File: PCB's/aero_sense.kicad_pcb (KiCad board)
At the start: 2 copper layers, 115 x 58 mm, 115 parts, among them J1 10164228-0201A1RLF, J10 10164227-0205A1RLF, J2 10164228-0201A1RLF, J3 10164228-0201A1RLF, J4 10164228-0201A1RLF, J5 10164227-0205A1RLF, J6 10164227-0205A1RLF, J7 Conn_01x04_Pin, J8 10164227-0205A1RLF, J9 USB4081-03-A_REV0.1, U10 TS3USB221DRCR, U11 KLM8G1GETF-B041, U12 STM32F417IGH6, U2 ICM-42688-P, U3 BMP581, U4 SGP41-D-R4, U5 SHT45-AD1F-R2, U7 SAM-M10Q-00B, U8 BQ25895RTWR, U9 AP2112K-3.3TRG1

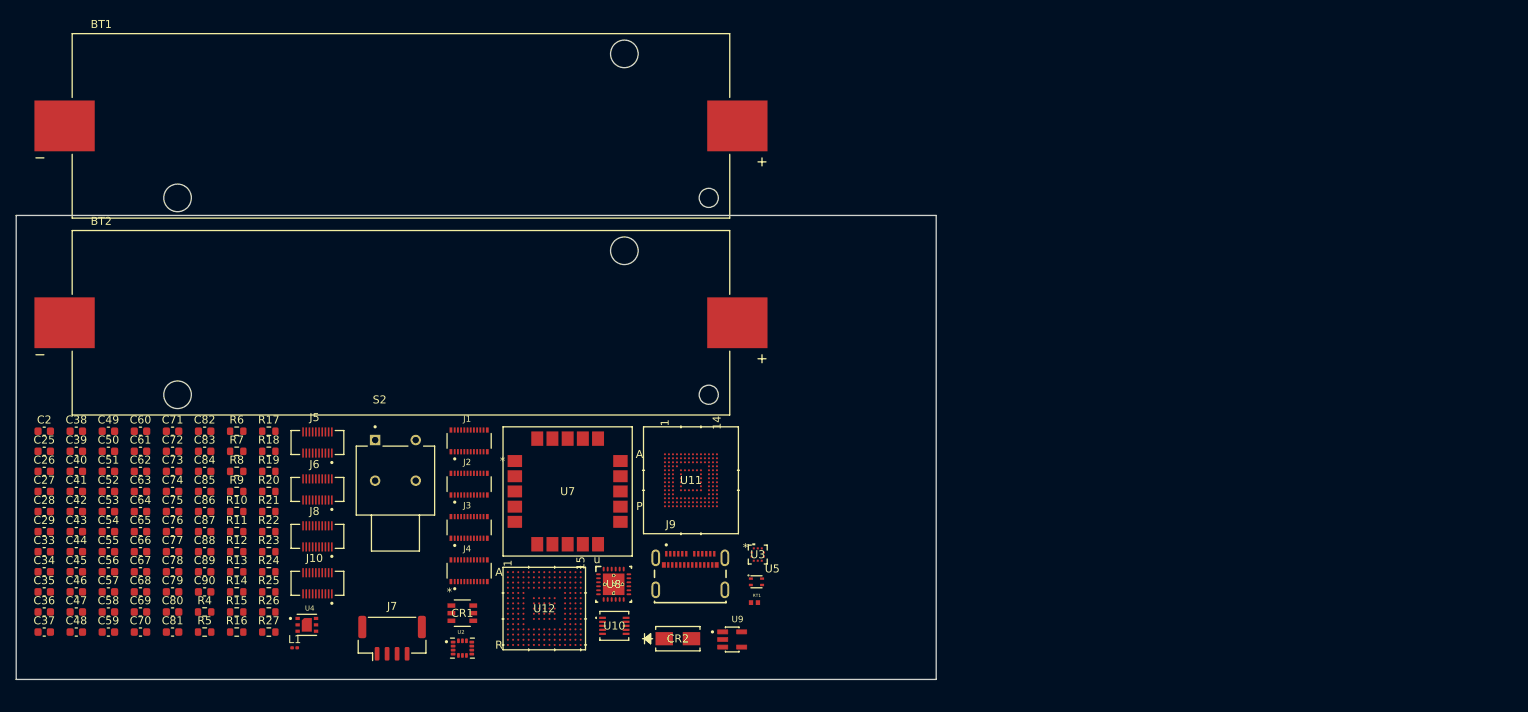
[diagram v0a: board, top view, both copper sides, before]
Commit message: unfinished changes
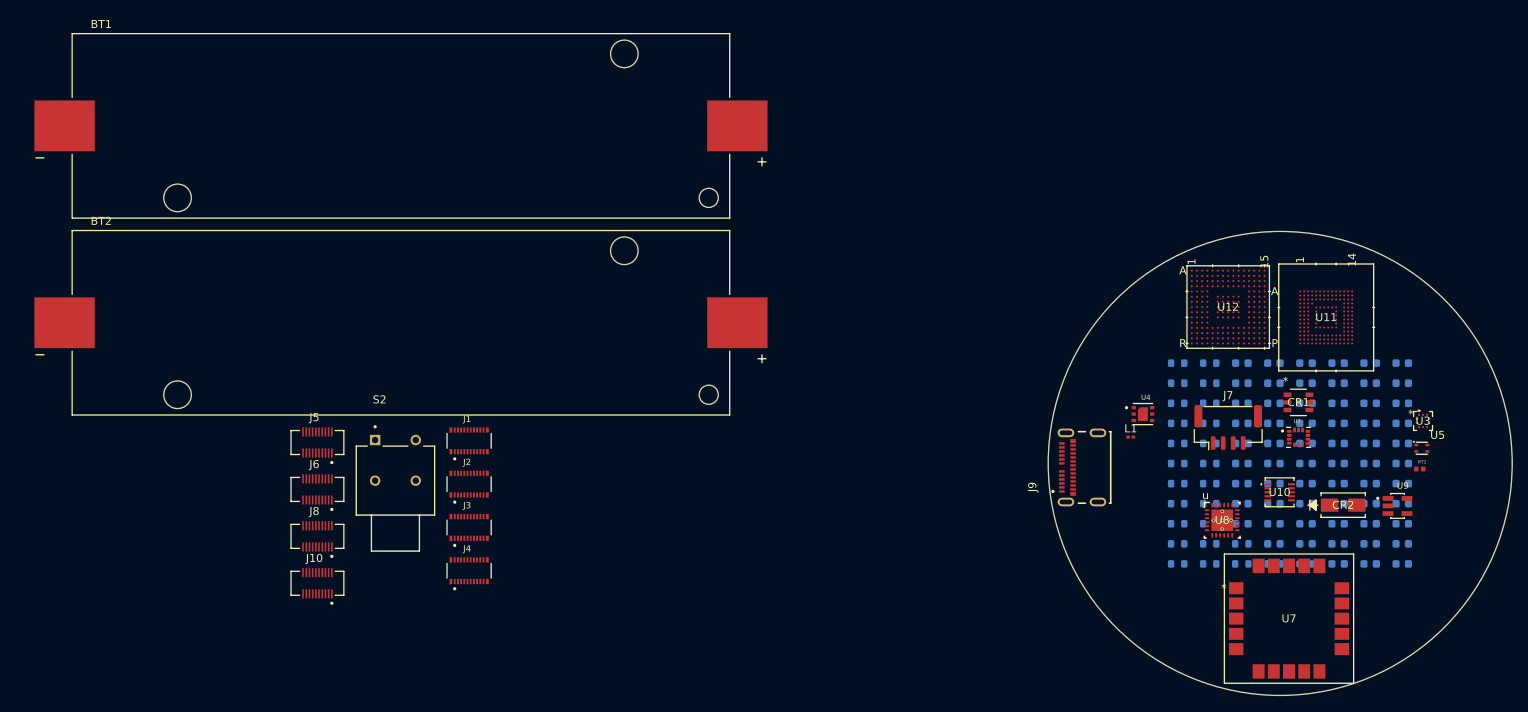
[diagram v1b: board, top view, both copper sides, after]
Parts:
- C2, C25, C26, C27, C28, C29, C33, C34, C35, C36, C37, C38, C39, C40, C41, C42, C43, C44, C45, C46, C47, C48, C49, C50, C51, C52, C53, C54, C55, C56, C57, C58, C59, C60, C61, C62, C63, C64, C65, C66, C67, C68, C69, C70, C71, C72, C73, C74, C75, C76, C77, C78, C79, C80, C81, C82, C83, C84, C85, C86, C87, C88, C89, C90, R10, R11, R12, R13, R14, R15, R16, R17, R18, R19, R20, R21, R22, R23, R24, R25, R26, R27, R4, R5, R6, R7, R8, R9: moved to B.Cu
- moved C2 170.0 mm to (235.3, 87.0), turned to 180 degrees
- moved C25 170.0 mm to (235.3, 89.5), turned to 180 degrees
- moved C26 170.0 mm to (235.3, 92.0), turned to 180 degrees
- moved C27 170.0 mm to (235.3, 94.5), turned to 180 degrees
- moved C28 170.0 mm to (235.3, 97.0), turned to 180 degrees
- moved C29 170.0 mm to (235.3, 99.5), turned to 180 degrees
- moved C33 170.0 mm to (235.3, 102.0), turned to 180 degrees
- moved C34 170.0 mm to (235.3, 104.5), turned to 180 degrees
- moved C35 170.0 mm to (235.3, 107.0), turned to 180 degrees
- moved C36 170.0 mm to (235.3, 109.5), turned to 180 degrees
- moved C37 170.0 mm to (235.3, 112.1), turned to 180 degrees
- moved C38 162.0 mm to (231.2, 87.0), turned to 180 degrees
- moved C39 162.0 mm to (231.2, 89.5), turned to 180 degrees
- moved C40 162.0 mm to (231.2, 92.0), turned to 180 degrees
- moved C41 162.0 mm to (231.2, 94.5), turned to 180 degrees
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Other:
- board size 115 x 58 mm -> 58 x 58 mm
